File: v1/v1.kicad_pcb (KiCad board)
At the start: 2 copper layers, 48.3 x 30.5 mm, 10 parts, among them J3 PWR, J4 RGB, U1 WeMos_D1_mini, U2 LevelShifter

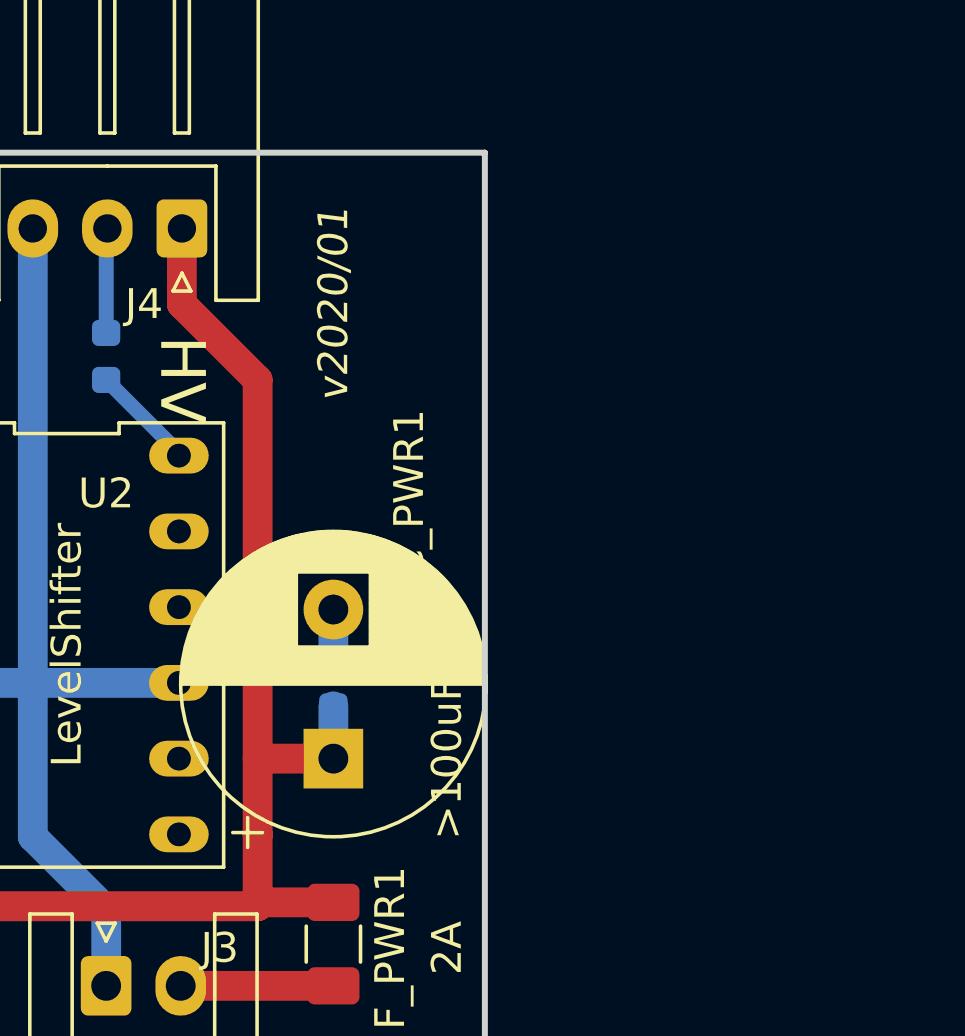
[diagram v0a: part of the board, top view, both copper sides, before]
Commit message: angled capacitor
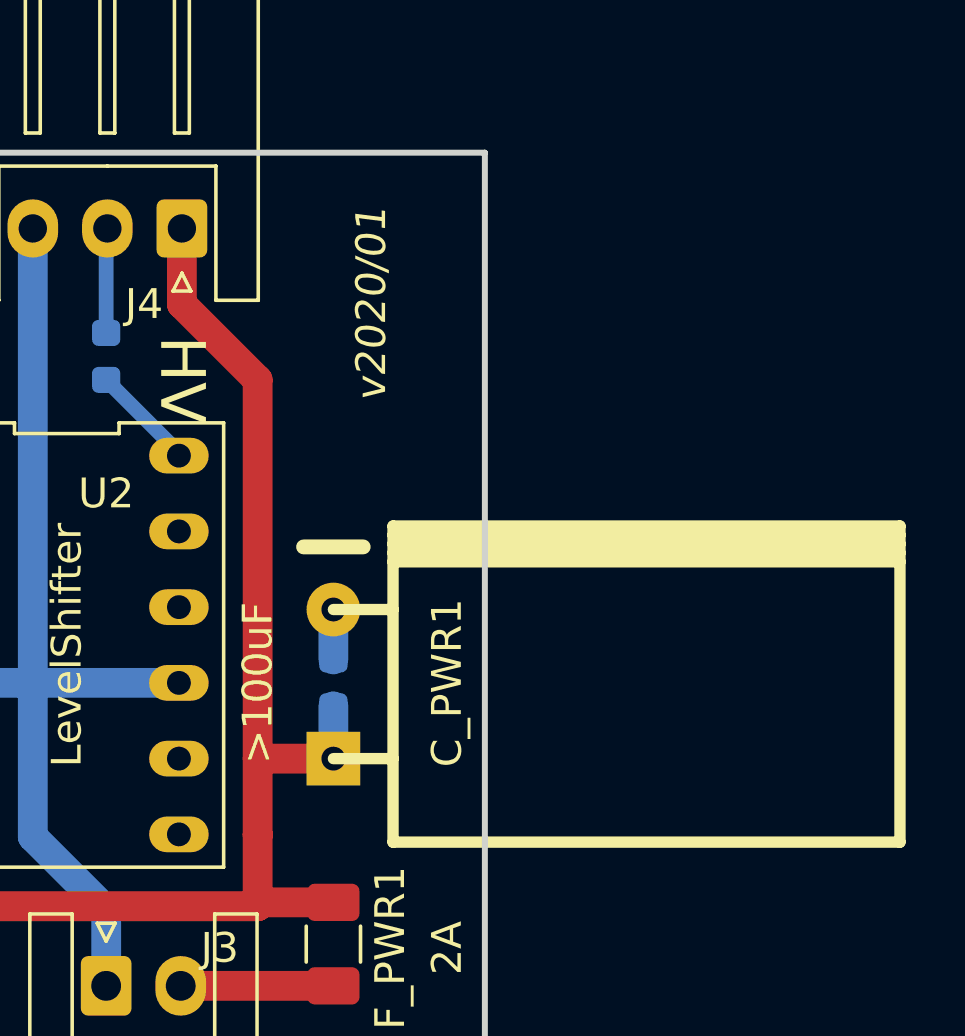
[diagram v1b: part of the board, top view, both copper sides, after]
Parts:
- C_PWR1: footprint Capacitor_THT:CP_Radial_D10.0mm_P5.00mm -> w_capacitors:CP_10x16mm_hor
- moved C_PWR1 9.63 mm to (105.8, 68.6), turned to 0 degrees
